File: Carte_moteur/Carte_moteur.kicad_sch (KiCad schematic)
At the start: 15 parts, among them J101 Conn_01x02_Socket, J102 Conn_01x02, J103 Conn_01x02, J104 Conn_01x07, U101 LD1117S33TR_SOT223

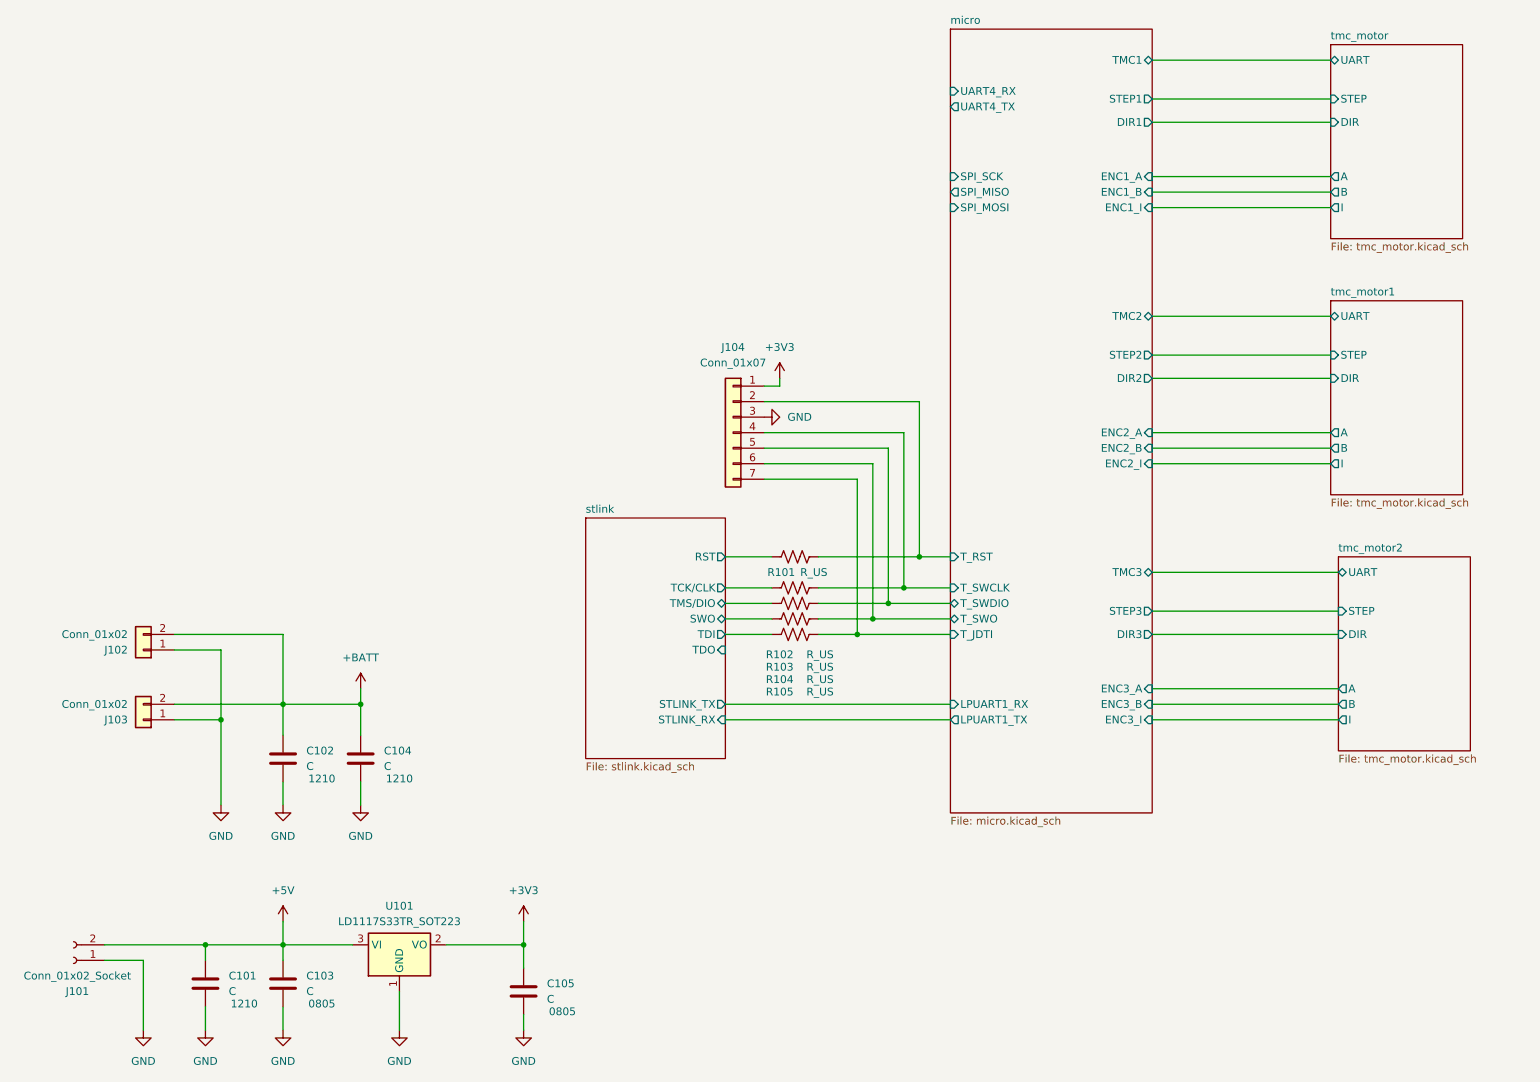
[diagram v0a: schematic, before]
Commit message: updated motor PCB
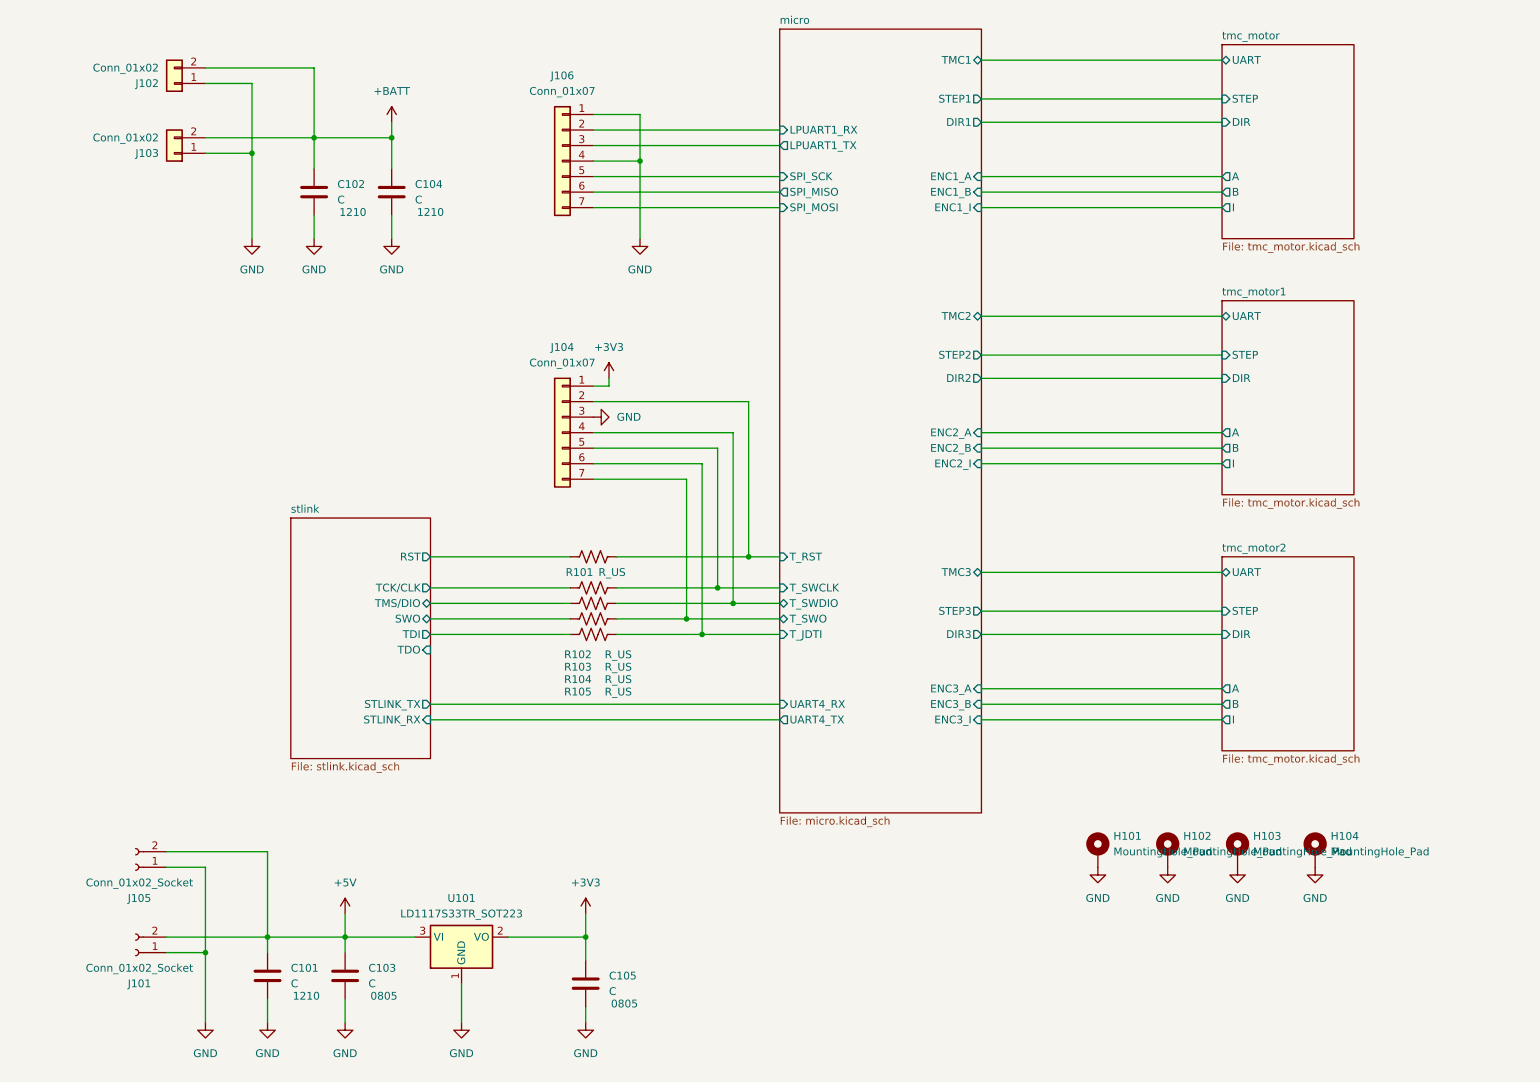
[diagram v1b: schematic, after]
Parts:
- added H101, H102, H103, H104: MountingHole_Pad, MountingHole:MountingHole_3.2mm_M3_DIN965_Pad, symbol Mechanical:MountingHole_Pad
- added J105: Conn_01x02_Socket, Connector_Molex:Molex_KK-396_A-41791-0002_1x02_P3.96mm_Vertical, symbol Connector:Conn_01x02_Socket
- added J106: Conn_01x07, Connector_Molex:Molex_KK-254_AE-6410-07A_1x07_P2.54mm_Vertical, symbol Connector_Generic:Conn_01x07
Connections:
- net +5V: now also J105.2 (Pin_2)
- net GND: now also H101.1, H102.1, H103.1, H104.1, J105.1 (Pin_1), J106.1 (Pin_1), J106.4 (Pin_4)
- net micro/LPUART1_RX: now also J106.2 (Pin_2)
- net micro/LPUART1_TX: now also J106.3 (Pin_3)
- net micro/SPI_MISO: now also J106.6 (Pin_6)
- net micro/SPI_MOSI: now also J106.7 (Pin_7)
- net micro/SPI_SCK: now also J106.5 (Pin_5)
- net micro/T_JDTI: now also J104.6 (Pin_6); no longer J104.7 (Pin_7)
- net micro/T_SWCLK: now also J104.5 (Pin_5); no longer J104.4 (Pin_4)
- net micro/T_SWDIO: now also J104.4 (Pin_4); no longer J104.5 (Pin_5)
- net micro/T_SWO: now also J104.7 (Pin_7); no longer J104.6 (Pin_6)
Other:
- moved on the sheet: C101, C102, C103, C104, C105, J101, J102, J103, J104, R101, R102, R103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
